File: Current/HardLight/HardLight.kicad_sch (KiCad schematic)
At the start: 59 parts, among them J0 USB, J1 qwiic, J2 Expansion, U0 RP2040, U1 MT2492, U2 USBLC6-2SC6, U3 W25Q128JVS, Y0 CSTCE12M0G55-R0

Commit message: Final Warning begins. Sweet Business done.
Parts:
- J2: footprint Connector_PinHeader_1.27mm:PinHeader_1x06_P1.27mm_Vertical -> Connector_PinHeader_2.54mm:PinHeader_1x06_P2.54mm_Vertical

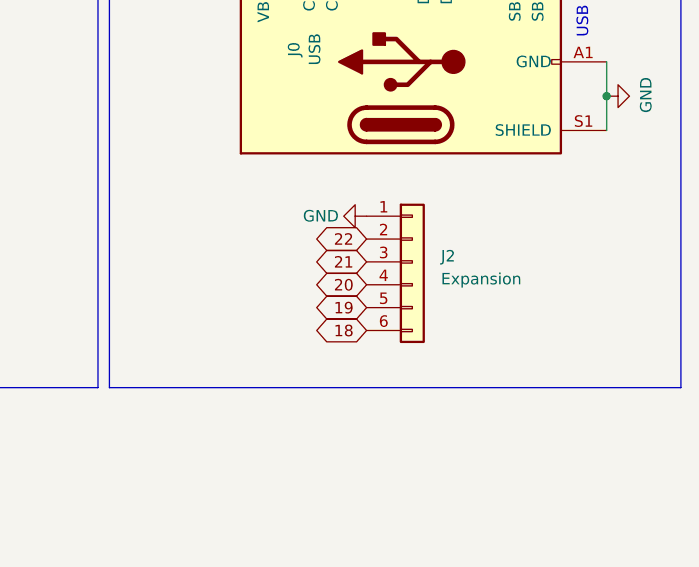
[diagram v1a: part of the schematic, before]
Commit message: Updates to Hardlight, to EDI footprint gallery
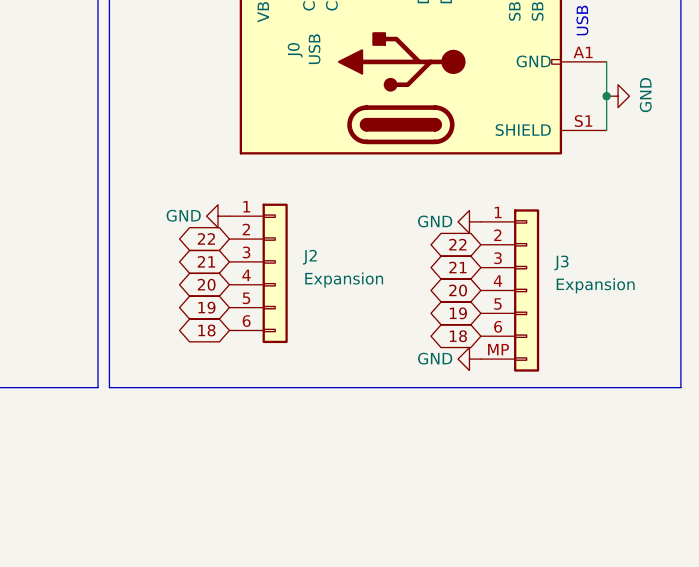
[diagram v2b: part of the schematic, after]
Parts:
- added J3: Expansion, Connector_JST:JST_SH_SM06B-SRSS-TB_1x06-1MP_P1.00mm_Horizontal, symbol Connector_Generic:Conn_01x06
- TX0, TX1: LCSC C391035 -> C255319
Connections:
- net 18: now also J3.6 (Pin_6)
- net 19: now also J3.5 (Pin_5)
- net 20: now also J3.4 (Pin_4)
- net 21: now also J3.3 (Pin_3)
- net 22: now also J3.2 (Pin_2)
- net GND: now also J3.1 (Pin_1), J3.MP (Mount_Point)
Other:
- moved on the sheet: J2
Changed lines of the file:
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@@
     (effects (font (size 1.27 1.27)) (justify right bottom))
   )
+  (global_label "18" (shape bidirectional) (at 240.665 162.56 180) (fields_autoplaced)
+    (effects (font (size 1.27 1.27)) (justify right))
+    (property "Intersheetrefs" "${INTERSHEET_REFS}" (at 235.9218 162.6394 0)
+      (effects (font (size 1.27 1.27)) (justify right) hide)
+    )
+  )
   (global_label "vUSB" (shape input) (at 216.535 116.84 180) (fields_autoplaced)
     (effects (font (size 1.27 1.27)) (justify right))
@@
     )
   )
+  (global_label "22" (shape bidirectional) (at 240.665 152.4 180) (fields_autoplaced)
+    (effects (font (size 1.27 1.27)) (justify right))
+    (property "Intersheetrefs" "${INTERSHEET_REFS}" (at 235.9218 152.4794 0)
+      (effects (font (size 1.27 1.27)) (justify right) hide)
+    )
+  )
   (global_label "col1" (shape output) (at 135.255 38.735 0) (fields_autoplaced)
     (effects (font (size 1.27 1.27)) (justify left))
@@
     )
   )
-  (global_label "22" (shape bidirectional) (at 227.965 151.765 180) (fields_autoplaced)
+  (global_label "19" (shape bidirectional) (at 240.665 160.02 180) (fields_autoplaced)
+    (effects (font (size 1.27 1.27)) (justify right))
+    (property "Intersheetrefs" "${INTERSHEET_REFS}" (at 235.9218 160.0994 0)
+      (effects (font (size 1.27 1.27)) (justify right) hide)
+    )
+  )
+  (global_label "22" (shape bidirectional) (at 212.725 151.765 180) (fields_autoplaced)
     (effects (font (size 1.27 1.27)) (justify right))
-    (property "Intersheetrefs" "${INTERSHEET_REFS}" (at 223.2218 151.8444 0)
+    (property "Intersheetrefs" "${INTERSHEET_REFS}" (at 207.9818 151.8444 0)
       (effects (font (size 1.27 1.27)) (justify right) hide)
     )
   )
-  (global_label "19" (shape bidirectional) (at 227.965 159.385 180) (fields_autoplaced)
+  (global_label "19" (shape bidirectional) (at 212.725 159.385 180) (fields_autoplaced)
     (effects (font (size 1.27 1.27)) (justify right))
-    (property "Intersheetrefs" "${INTERSHEET_REFS}" (at 223.2218 159.4644 0)
+    (property "Intersheetrefs" "${INTERSHEET_REFS}" (at 207.9818 159.4644 0)
       (effects (font (size 1.27 1.27)) (justify right) hide)
     )
@@
     )
   )
-  (global_label "20" (shape bidirectional) (at 227.965 156.845 180) (fields_autoplaced)
+  (global_label "20" (shape bidirectional) (at 240.665 157.48 180) (fields_autoplaced)
+    (effects (font (size 1.27 1.27)) (justify right))
+    (property "Intersheetrefs" "${INTERSHEET_REFS}" (at 235.9218 157.5594 0)
+      (effects (font (size 1.27 1.27)) (justify right) hide)
+    )
+  )
+  (global_label "20" (shape bidirectional) (at 212.725 156.845 180) (fields_autoplaced)
     (effects (font (size 1.27 1.27)) (justify right))
-    (property "Intersheetrefs" "${INTERSHEET_REFS}" (at 223.2218 156.9244 0)
+    (property "Intersheetrefs" "${INTERSHEET_REFS}" (at 207.9818 156.9244 0)
       (effects (font (size 1.27 1.27)) (justify right) hide)
     )
@@
     )
   )
-  (global_label "18" (shape bidirectional) (at 227.965 161.925 180) (fields_autoplaced)
+  (global_label "18" (shape bidirectional) (at 212.725 161.925 180) (fields_autoplaced)
     (effects (font (size 1.27 1.27)) (justify right))
-    (property "Intersheetrefs" "${INTERSHEET_REFS}" (at 223.2218 162.0044 0)
+    (property "Intersheetrefs" "${INTERSHEET_REFS}" (at 207.9818 162.0044 0)
       (effects (font (size 1.27 1.27)) (justify right) hide)
     )
@@
     )
   )
-  (global_label "21" (shape bidirectional) (at 227.965 154.305 180) (fields_autoplaced)
+  (global_label "21" (shape bidirectional) (at 212.725 154.305 180) (fields_autoplaced)
     (effects (font (size 1.27 1.27)) (justify right))
-    (property "Intersheetrefs" "${INTERSHEET_REFS}" (at 223.2218 154.3844 0)
+    (property "Intersheetrefs" "${INTERSHEET_REFS}" (at 207.9818 154.3844 0)
       (effects (font (size 1.27 1.27)) (justify right) hide)
     )
@@
     )
   )
+  (global_label "21" (shape bidirectional) (at 240.665 154.94 180) (fields_autoplaced)
+    (effects (font (size 1.27 1.27)) (justify right))
+    (property "Intersheetrefs" "${INTERSHEET_REFS}" (at 235.9218 155.0194 0)
+      (effects (font (size 1.27 1.27)) (justify right) hide)
+    )
+  )
   (global_label "col4" (shape output) (at 135.255 46.355 0) (fields_autoplaced)
     (effects (font (size 1.27 1.27)) (justify left))
@@
       (effects (font (size 1.27 1.27)) hide)
     )
-    (property "LCSC" "C391035" (at 179.07 94.615 0)
+    (property "LCSC" "C255319" (at 179.07 94.615 0)
       (effects (font (size 1.27 1.27)) hide)
     )
@@
       (effects (font (size 1.27 1.27)) hide)
     )
-    (property "LCSC" "C391035" (at 179.07 111.125 0)
+    (property "LCSC" "C255319" (at 179.07 111.125 0)
       (effects (font (size 1.27 1.27)) hide)
     )
@@
     )
   )
-  (symbol (lib_id "power:GND") (at 227.965 149.225 270) (unit 1)
+  (symbol (lib_id "power:GND") (at 212.725 149.225 270) (unit 1)
     (in_bom yes) (on_board yes) (dnp no)
-    (property "Reference" "#PWR014" (at 221.615 149.225 0)
+    (property "Reference" "#PWR014" (at 206.375 149.225 0)
       (effects (font (size 1.27 1.27)) hide)
     )
-    (property "Value" "GND" (at 222.885 149.225 90)
+    (property "Value" "GND" (at 207.645 149.225 90)
       (effects (font (size 1.27 1.27)))
     )
-    (property "Footprint" "" (at 227.965 149.225 0)
+    (property "Footprint" "" (at 212.725 149.225 0)
       (effects (font (size 1.27 1.27)) hide)
     )
-    (property "Datasheet" "" (at 227.965 149.225 0)
+    (property "Datasheet" "" (at 212.725 149.225 0)
       (effects (font (size 1.27 1.27)) hide)
     )
@@
     )
   )
+  (symbol (lib_id "power:GND") (at 240.665 149.86 270) (unit 1)
+    (in_bom yes) (on_board yes) (dnp no)
+    (property "Reference" "#PWR015" (at 234.315 149.86 0)
+      (effects (font (size 1.27 1.27)) hide)
+    )
+    (property "Value" "GND" (at 235.585 149.86 90)
+      (effects (font (size 1.27 1.27)))
+    )
+    (property "Footprint" "" (at 240.665 149.86 0)
+      (effects (font (size 1.27 1.27)) hide)
+    )
+    (property "Datasheet" "" (at 240.665 149.86 0)
+      (effects (font (size 1.27 1.27)) hide)
+    )
+    (pin "1")
+    (instances
+      (project "HardLight"
+        (path "/bd065eaf-e495-4837-bdb3-129934de1fc7"
+          (reference "#PWR015") (unit 1)
+        )
+      )
+    )
+  )
   (symbol (lib_id "Device:C_Small") (at 50.8 190.5 0) (unit 1)
     (in_bom yes) (on_board yes) (dnp no)
@@
     )
   )
+  (symbol (lib_id "power:GND") (at 240.665 165.1 270) (unit 1)
+    (in_bom yes) (on_board yes) (dnp no)
+    (property "Reference" "#PWR016" (at 234.315 165.1 0)
+      (effects (font (size 1.27 1.27)) hide)
+    )
+    (property "Value" "GND" (at 235.585 165.1 90)
+      (effects (font (size 1.27 1.27)))
+    )
+    (property "Footprint" "" (at 240.665 165.1 0)
+      (effects (font (size 1.27 1.27)) hide)
+    )
+    (property "Datasheet" "" (at 240.665 165.1 0)
+      (effects (font (size 1.27 1.27)) hide)
+    )
+    (pin "1")
+    (instances
+      (project "HardLight"
+        (path "/bd065eaf-e495-4837-bdb3-129934de1fc7"
+          (reference "#PWR016") (unit 1)
+        )
+      )
+    )
+  )
   (symbol (lib_id "Mechanical:MountingHole") (at 172.72 163.83 270) (unit 1)
     (in_bom yes) (on_board yes) (dnp no)
@@
     )
   )
+  (symbol (lib_name "Conn_01x06_1") (lib_id "Connector_Generic:Conn_01x06") (at 245.745 154.94 0) (unit 1)
+    (in_bom yes) (on_board yes) (dnp no) (fields_autoplaced)
+    (property "Reference" "J3" (at 248.92 154.305 0)
+      (effects (font (size 1.27 1.27)) (justify left))
+    )
+    (property "Value" "Expansion" (at 248.92 156.845 0)
+      (effects (font (size 1.27 1.27)) (justify left))
+    )
+    (property "Footprint" "Connector_JST:JST_SH_SM06B-SRSS-TB_1x06-1MP_P1.00mm_Horizontal" (at 245.745 154.94 0)
+      (effects (font (size 1.27 1.27)) hide)
+    )
+    (property "Datasheet" "~" (at 245.745 154.94 0)
+      (effects (font (size 1.27 1.27)) hide)
+    )
+    (property "LCSC" " C5175296" (at 245.745 154.94 0)
+      (effects (font (size 1.27 1.27)) hide)
+    )
+    (pin "1")
+    (pin "2")
+    (pin "3")
+    (pin "4")
+    (pin "5")
+    (pin "6")
+    (pin "MP")
+    (instances
+      (project "HardLight"
+        (path "/bd065eaf-e495-4837-bdb3-129934de1fc7"
+          (reference "J3") (unit 1)
+        )
+      )
+    )
+  )
   (symbol (lib_id "Device:C_Small") (at 58.547 157.48 0) (unit 1)
     (in_bom yes) (on_board yes) (dnp no)
@@
     )
   )
-  (symbol (lib_id "Connector_Generic:Conn_01x06") (at 233.045 154.305 0) (unit 1)
+  (symbol (lib_id "Connector_Generic:Conn_01x06") (at 217.805 154.305 0) (unit 1)
     (in_bom yes) (on_board yes) (dnp no) (fields_autoplaced)
-    (property "Reference" "J2" (at 236.22 153.67 0)
+    (property "Reference" "J2" (at 220.98 153.67 0)
       (effects (font (size 1.27 1.27)) (justify left))
     )
-    (property "Value" "Expansion" (at 236.22 156.21 0)
+    (property "Value" "Expansion" (at 220.98 156.21 0)
       (effects (font (size 1.27 1.27)) (justify left))
     )
-    (property "Footprint" "Connector_PinHeader_2.54mm:PinHeader_1x06_P2.54mm_Vertical" (at 233.045 154.305 0)
+    (property "Footprint" "Connector_PinHeader_2.54mm:PinHeader_1x06_P2.54mm_Vertical" (at 217.805 154.305 0)
       (effects (font (size 1.27 1.27)) hide)
     )
-    (property "Datasheet" "~" (at 233.045 154.305 0)
+    (property "Datasheet" "~" (at 217.805 154.305 0)
       (effects (font (size 1.27 1.27)) hide)
     )
